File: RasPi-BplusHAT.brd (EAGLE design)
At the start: 65 x 56 mm, 10 parts, among them K1 PIN20X2

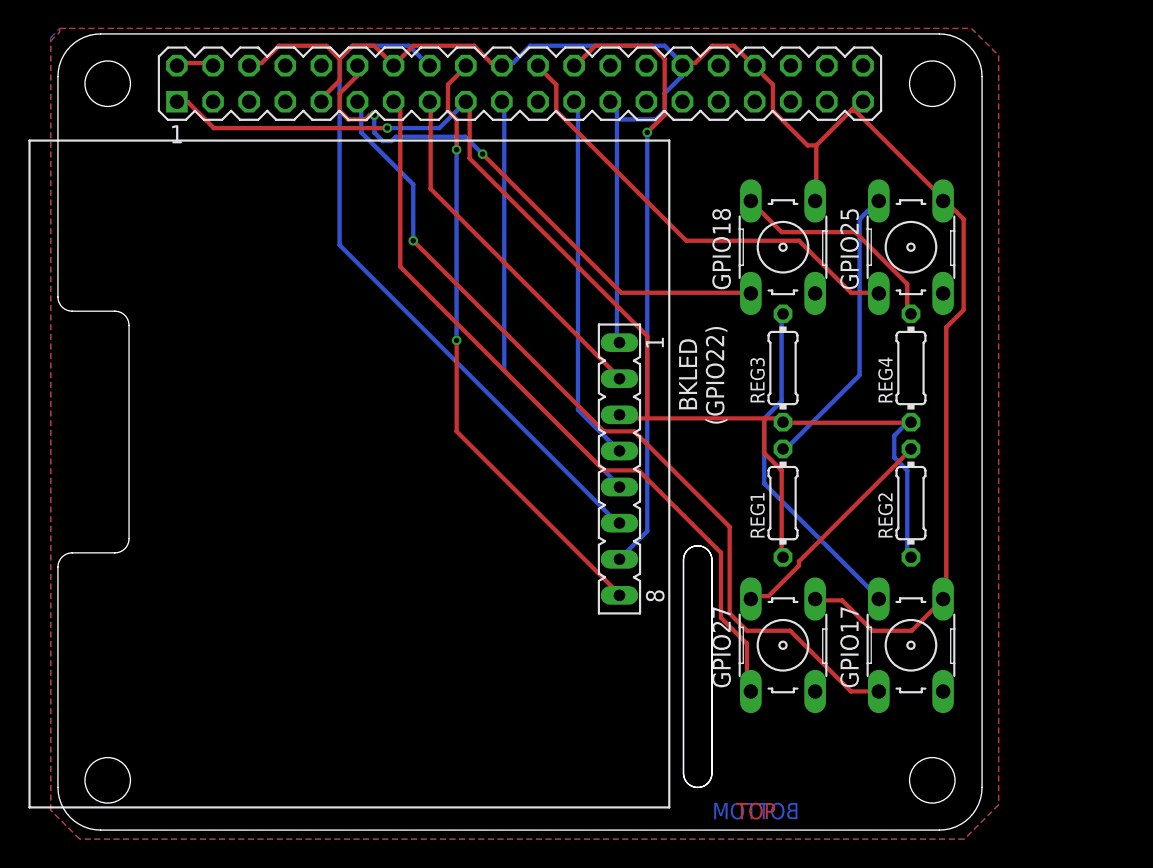
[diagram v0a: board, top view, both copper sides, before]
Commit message: Auto routed
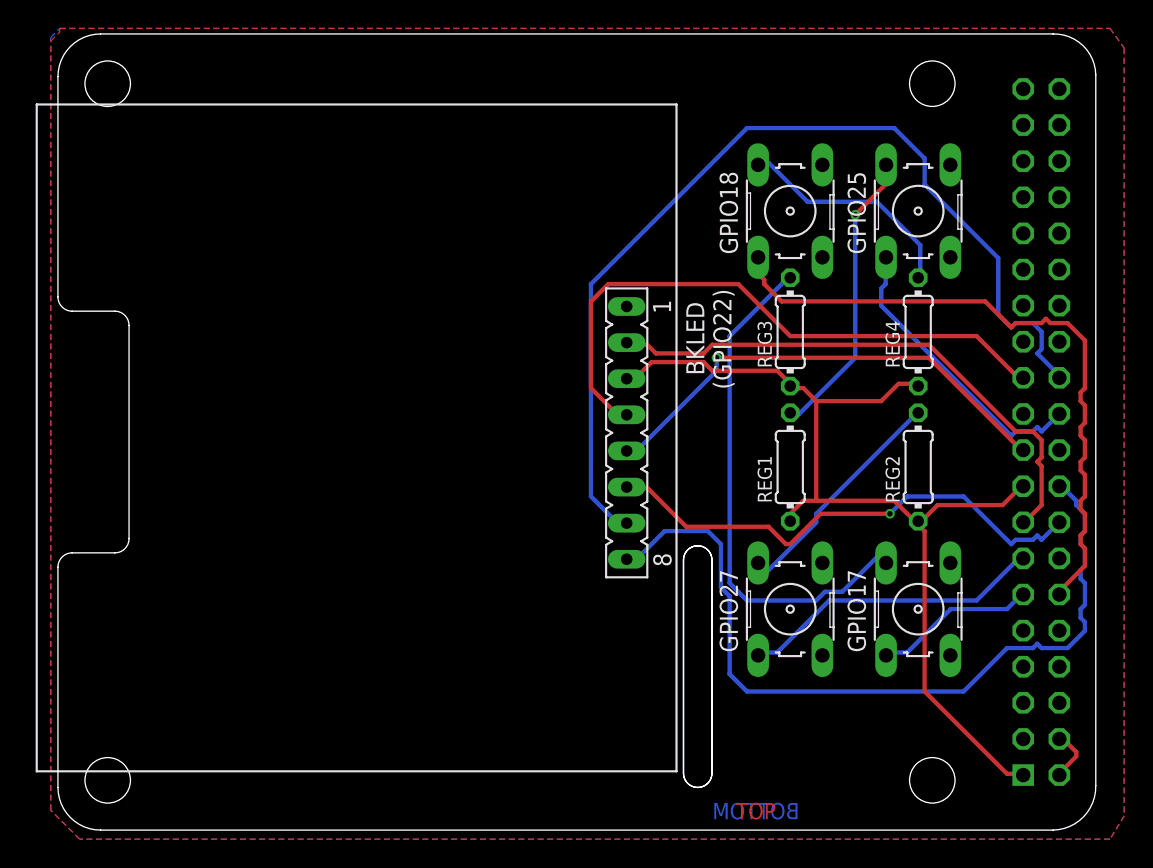
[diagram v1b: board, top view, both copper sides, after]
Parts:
- moved K1 44.1 mm to (69.2, 28.0), flipped to the bottom, turned to 90 degrees
- moved SV1 2.59 mm to (40.0, 27.9)
- moved GPIO17 2.59 mm to (60.5, 15.5)
- moved GPIO18 2.59 mm to (51.5, 43.5)
- moved GPIO25 2.59 mm to (60.5, 43.5)
- moved GPIO27 2.59 mm to (51.5, 15.5)
- moved REG1 2.59 mm to (51.5, 25.5)
- moved REG2 2.59 mm to (60.5, 25.5)
- moved REG3 2.59 mm to (51.5, 35.0)
- moved REG4 2.59 mm to (60.5, 35.0)
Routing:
- net GND: track 134.7 -> 0.00 mm
- net BUTTON2: track 61.0 -> 11.7 mm, vias 1 -> 0
- net BUTTON3: track 53.5 -> 21.6 mm
- net CE: track 43.8 -> 68.0 mm, vias 1 -> 0
- net +3V3: track 91.5 -> 70.6 mm, vias 1 -> 0
- net CLK: track 26.0 -> 43.1 mm
- net BL: track 25.0 -> 39.1 mm
- net RESET: track 42.8 -> 56.6 mm, vias 2 -> 0
- net DC: track 48.2 -> 35.7 mm, vias 0 -> 1
- net N$3: track 24.0 -> 36.3 mm
- net BUTTON4: track 31.7 -> 20.7 mm
- net BUTTON1: track 39.1 -> 46.7 mm, vias 2 -> 0
- net DIN: track 30.6 -> 34.0 mm, vias 0 -> 1
- net +5V: track 2.68 -> 3.82 mm
- net N$4: track 15.6 -> 16.2 mm
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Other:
- board size 65 x 56 mm -> 73 x 56 mm
